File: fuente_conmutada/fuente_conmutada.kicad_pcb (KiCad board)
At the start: 2 copper layers, 206 x 163.7 mm, 64 parts, among them J1 shutdown, J2 Conn_01x03, J3 Conn_01x03, J4 Conn_01x02, J5 Conn_01x02, J6 in_red, J7 out_12v, J8 out_pwr, U1 UC3525

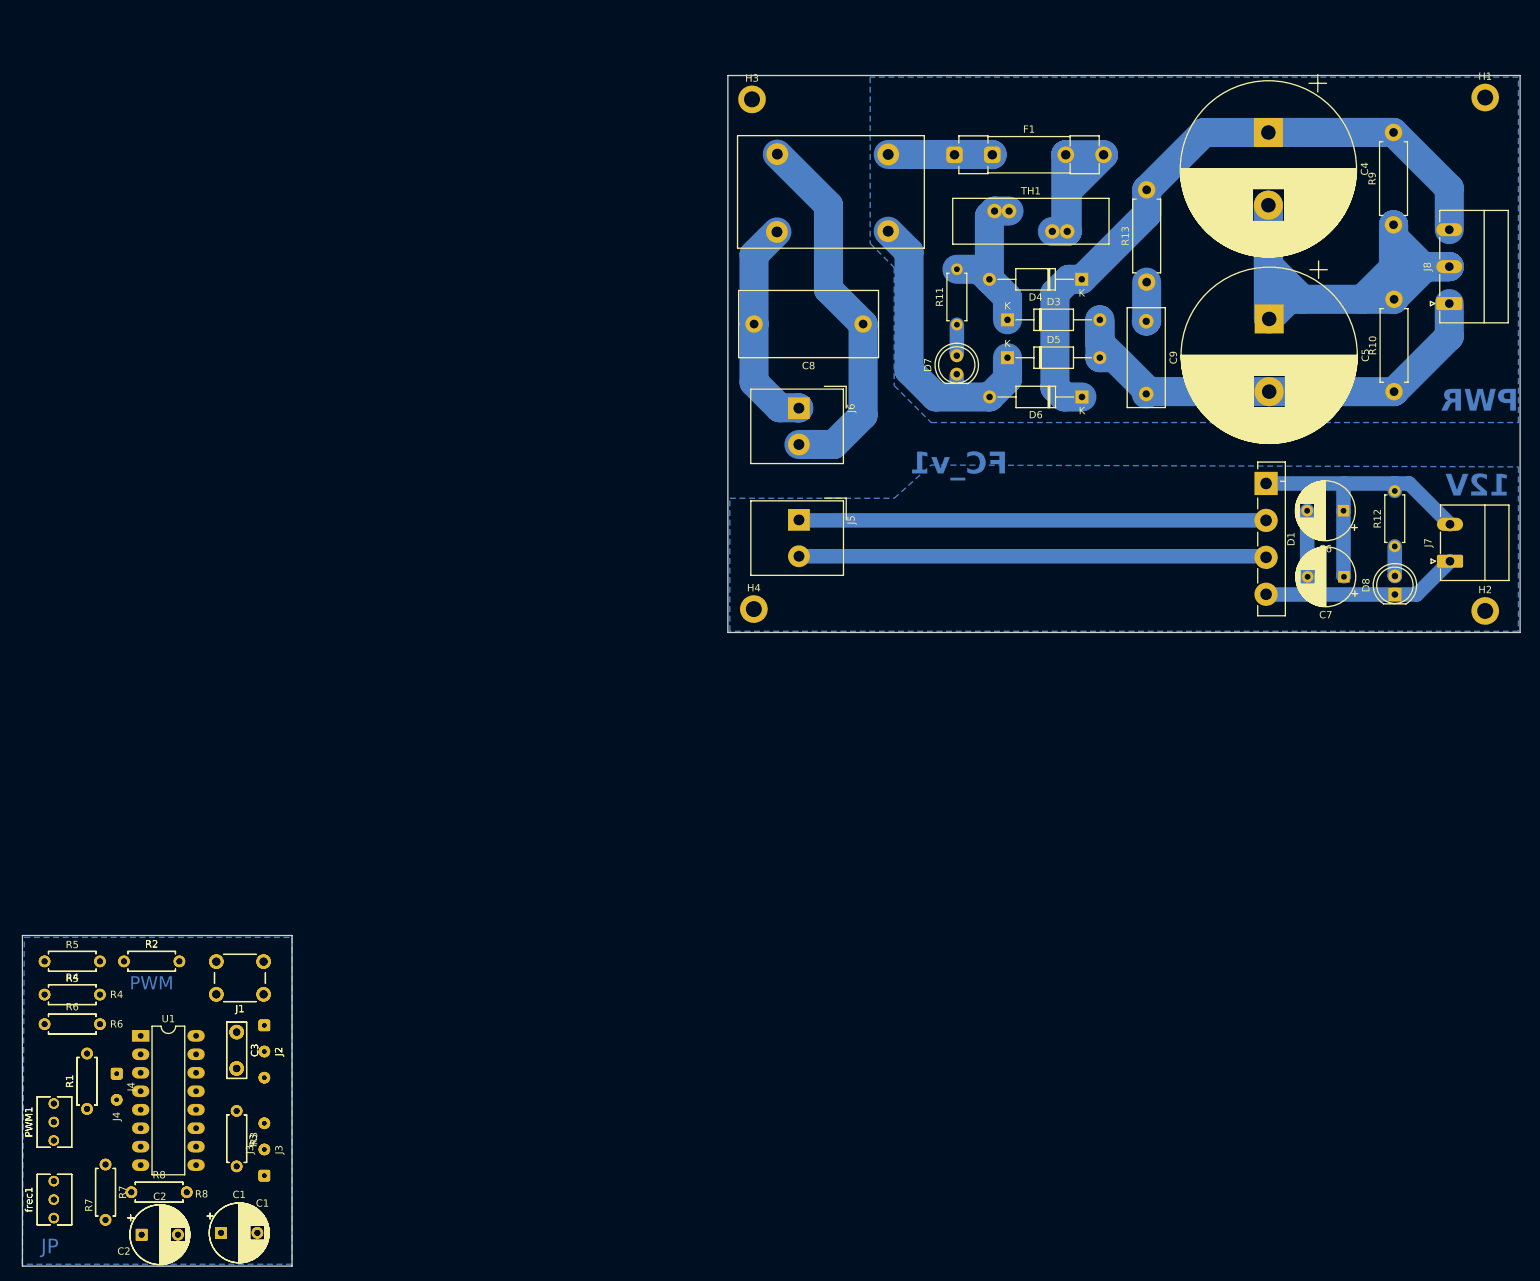
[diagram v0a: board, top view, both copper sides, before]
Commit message: fc_v1
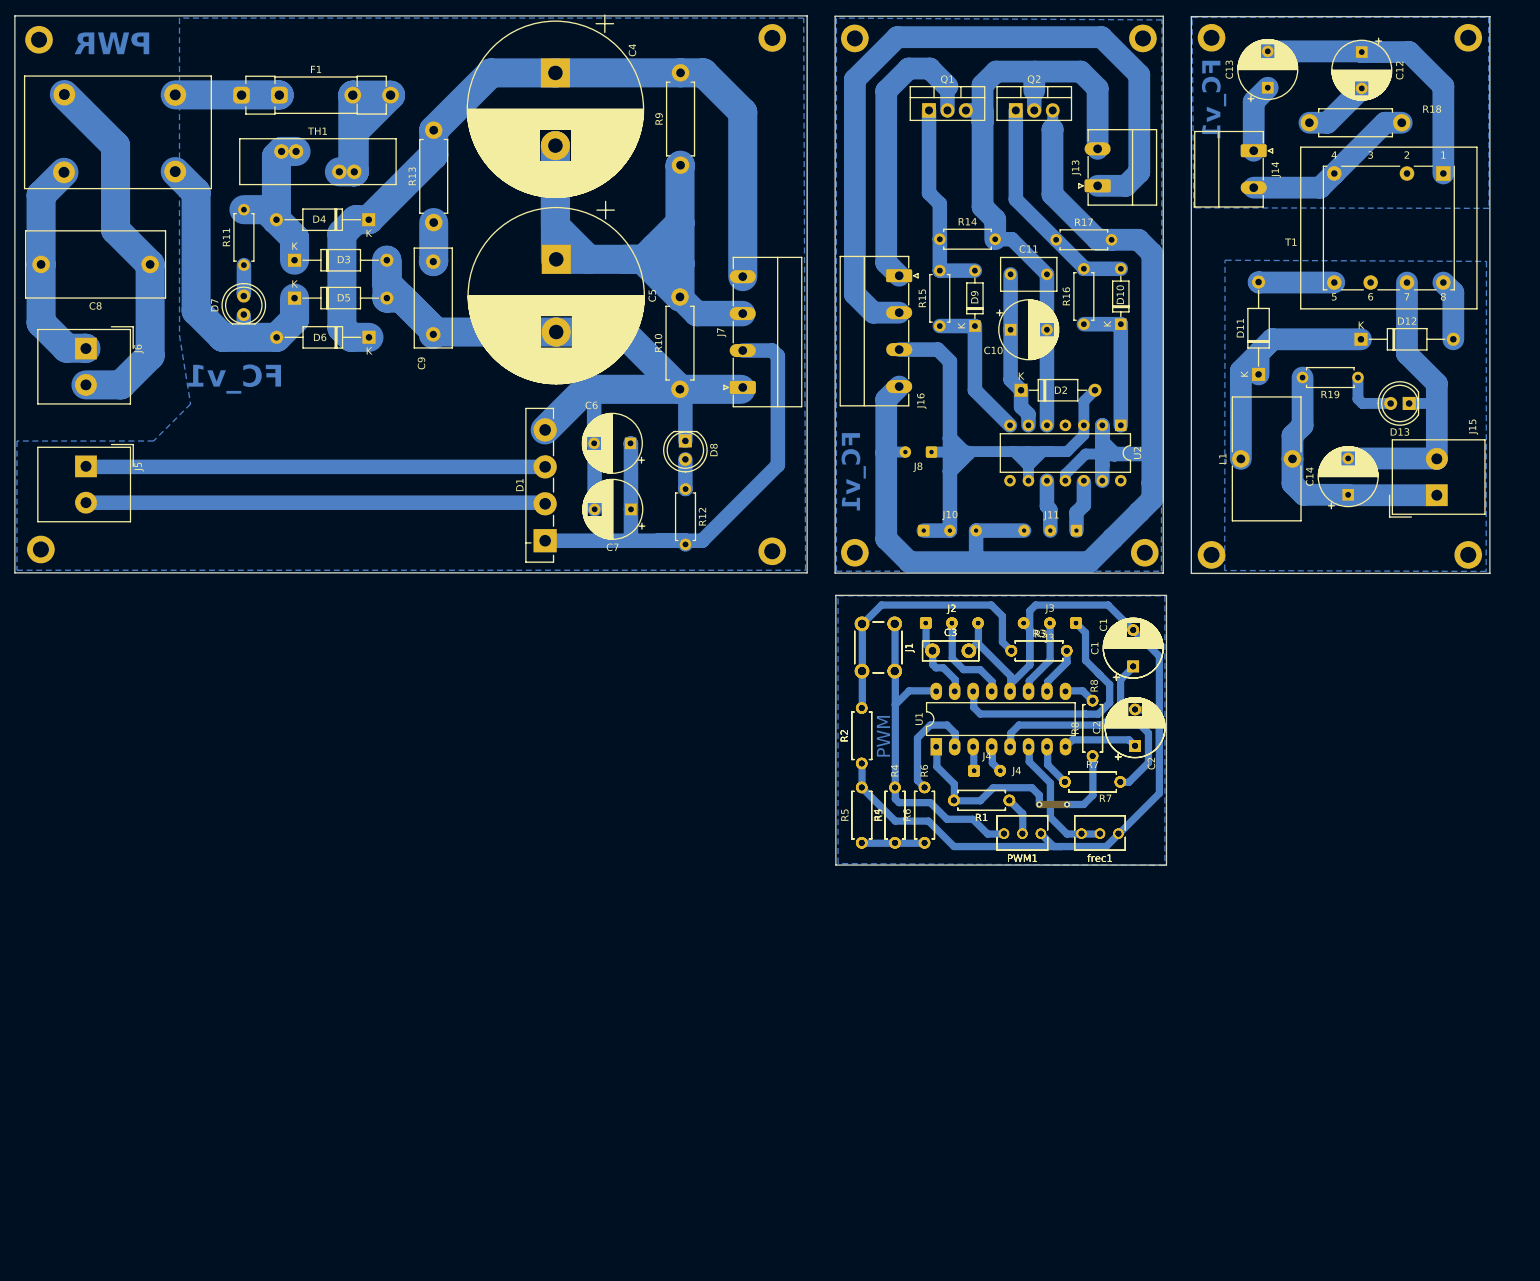
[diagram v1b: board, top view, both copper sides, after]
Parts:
- added C10: 100n, Capacitor_THT:CP_Radial_D8.0mm_P5.00mm, F.Cu at (156.2, 63.4)
- added C11: 22u, Capacitor_THT:C_Disc_D7.5mm_W4.4mm_P5.00mm, F.Cu at (156.2, 55.8)
- added C12: 100n, Capacitor_THT:CP_Radial_D8.0mm_P5.00mm, F.Cu at (204.5, 25.2)
- added C13: 100n, Capacitor_THT:CP_Radial_D8.0mm_P5.00mm, F.Cu at (191.6, 30.1)
- added C14: 100n, Capacitor_THT:CP_Radial_D8.0mm_P5.00mm, F.Cu at (202.6, 86.1)
- added D10: 1N4148, Diode_THT:D_DO-35_SOD27_P7.62mm_Horizontal, F.Cu at (171.4, 62.7)
- added D11: D, Diode_THT:D_A-405_P12.70mm_Horizontal, F.Cu at (190.3, 69.6)
- added D12: D, Diode_THT:D_A-405_P12.70mm_Horizontal, F.Cu at (204.4, 64.7)
- added D13: LED, LED_THT:LED_D5.0mm, F.Cu at (211.0, 73.6)
- added D2: D, Diode_THT:D_A-405_P10.16mm_Horizontal, F.Cu at (157.7, 71.8)
- added D9: 1N4148, Diode_THT:D_DO-35_SOD27_P7.62mm_Horizontal, F.Cu at (151.3, 62.9)
- added H10: MountingHole, MountingHole:MountingHole_2.2mm_M2_DIN965_Pad, F.Cu at (219.2, 23.3)
- added H11: MountingHole, MountingHole:MountingHole_2.2mm_M2_DIN965_Pad, F.Cu at (183.9, 94.4)
- added H12: MountingHole, MountingHole:MountingHole_2.2mm_M2_DIN965_Pad, F.Cu at (219.2, 94.4)
- added H5: MountingHole, MountingHole:MountingHole_2.2mm_M2_DIN965_Pad, F.Cu at (134.8, 94.1)
- added H6: MountingHole, MountingHole:MountingHole_2.2mm_M2_DIN965_Pad, F.Cu at (134.8, 23.4)
- added H7: MountingHole, MountingHole:MountingHole_2.2mm_M2_DIN965_Pad, F.Cu at (174.4, 23.4)
- added H8: MountingHole, MountingHole:MountingHole_2.2mm_M2_DIN965_Pad, F.Cu at (174.7, 94.1)
- added H9: MountingHole, MountingHole:MountingHole_2.2mm_M2_DIN965_Pad, F.Cu at (183.9, 23.3)
- added J10: pwm_power, Connector_Wire:SolderWire-0.1sqmm_1x03_P3.6mm_D0.4mm_OD1mm, F.Cu at (144.3, 91.1)
- added J11: pwm_señal, Connector_Wire:SolderWire-0.1sqmm_1x03_P3.6mm_D0.4mm_OD1mm, F.Cu at (165.3, 91.1)
- added J13: trafo, Connector_Phoenix_MC_HighVoltage:PhoenixContact_MC_1,5_2-G-5.08_1x02_P5.08mm_Horizontal, F.Cu at (168.2, 43.6)
- added J14: in_trafo, Connector_Phoenix_MC_HighVoltage:PhoenixContact_MC_1,5_2-G-5.08_1x02_P5.08mm_Horizontal, F.Cu at (189.7, 38.8)
- added J15: out_R, TerminalBlock_Altech:Altech_AK300_1x02_P5.00mm_45-Degree, F.Cu at (214.8, 86.2)
- added J16: in_pwr, Connector_Phoenix_MC_HighVoltage:PhoenixContact_MC_1,5_4-G-5.08_1x04_P5.08mm_Horizontal, F.Cu at (140.9, 56.0)
- added L1: L, Inductor_THT:L_Toroid_Vertical_L16.8mm_W9.2mm_P7.10mm_Vishay_TJ3, F.Cu at (187.9, 81.2)
- added Q1: IRF740, Package_TO_SOT_THT:TO-220-3_Vertical, F.Cu at (145.0, 33.3)
- added Q2: IRF740, Package_TO_SOT_THT:TO-220-3_Vertical, F.Cu at (156.9, 33.3)
- added R14: 1k, Resistor_THT:R_Axial_DIN0207_L6.3mm_D2.5mm_P7.62mm_Horizontal, F.Cu at (146.5, 51.0)
- added R15: 100, Resistor_THT:R_Axial_DIN0207_L6.3mm_D2.5mm_P7.62mm_Horizontal, F.Cu at (146.5, 62.9)
- added R16: 100, Resistor_THT:R_Axial_DIN0207_L6.3mm_D2.5mm_P7.62mm_Horizontal, F.Cu at (166.3, 62.7)
- added R17: 1k, Resistor_THT:R_Axial_DIN0207_L6.3mm_D2.5mm_P7.62mm_Horizontal, F.Cu at (162.5, 51.1)
- added R18: 150k, Resistor_THT:R_Axial_DIN0411_L9.9mm_D3.6mm_P12.70mm_Horizontal, F.Cu at (210.0, 35.0)
- added R19: 22k, Resistor_THT:R_Axial_DIN0207_L6.3mm_D2.5mm_P7.62mm_Horizontal, F.Cu at (204.0, 70.0)
- added T1: Transformer_1P_SS, Transformer_THT:Transformer_Breve_TEZ-22x24, F.Cu at (215.7, 41.9)
- added U2: IR2110, Package_DIP:DIP-14_W7.62mm, F.Cu at (171.4, 76.6)
- J7: value out_12v -> in_pwr; footprint Connector_Phoenix_MC_HighVoltage:PhoenixContact_MC_1,5_2-G-5.08_1x02_P5.08mm_Horizontal -> Connector_Phoenix_MC_HighVoltage:PhoenixContact_MC_1,5_4-G-5.08_1x04_P5.08mm_Horizontal
- J8: value out_pwr -> fan; footprint Connector_Phoenix_MC_HighVoltage:PhoenixContact_MC_1,5_3-G-5.08_1x03_P5.08mm_Horizontal -> Connector_Wire:SolderWire-0.1sqmm_1x02_P3.6mm_D0.4mm_OD1mm
- moved C2 152.3 mm to (173.3, 120.7), turned to 90 degrees (x2)
- moved frec1 149.2 mm to (166.0, 132.7), turned to 180 degrees (x2)
- moved C1 147.7 mm to (173.1, 109.7), turned to 90 degrees (x2)
- moved R8 145.2 mm to (167.5, 122.1), turned to 90 degrees (x2)
- moved R7 142.1 mm to (163.7, 125.6), turned to 0 degrees (x2)
- moved PWM1 135.8 mm to (155.3, 132.7), turned to 180 degrees (x2)
- moved J3 135.1 mm to (165.2, 103.8), turned to 180 degrees
- moved J3 135.0 mm to (165.2, 103.8), turned to 180 degrees
- moved R1 133.8 mm to (156.1, 128.2), turned to 180 degrees
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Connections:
- C3 pad 1: +12V -> Vc
- C5 pad 2: GNDPWR -> GND
- C6 pad 1: +12V -> Vc
- C7 pad 1: +12V -> Vc
- C9 pad 2: GNDPWR -> GND
- D1 pad 1: +12V -> Vc
- D1 pad 2: Net-(J5-Pin_1) -> Net-(J5-Pin_2)
- D1 pad 3: Net-(J5-Pin_2) -> Net-(J5-Pin_1)
- D3 pad 2: GNDPWR -> GND
- D5 pad 2: GNDPWR -> GND
- J2 pad 1: +12V -> Vc
- J7 pad 2: +12V -> Vc
- J8 pad 1: GNDPWR -> Vc
- J8 pad 2: 155V -> GND
- R10 pad 1: GNDPWR -> GND
- R12 pad 2: +12V -> Vc
- U1 pad 15: +12V -> Vc
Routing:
- net GND: track 38.7 -> 420.4 mm
- net Vc: track 0.00 -> 166.1 mm
- net 155V: track 108.8 -> 218.4 mm
- net VS: track 0.00 -> 96.4 mm
- net GNDPWR: track 76.0 -> 0.00 mm
- net 310V: track 91.5 -> 148.5 mm
- net Vref: track 0.00 -> 47.5 mm
- net OutB: track 0.00 -> 42.5 mm
- net GNDREF: track 0.00 -> 42.3 mm
- net Net-(U1-CT): track 0.00 -> 41.0 mm
- net Net-(T1-AA): track 0.00 -> 38.1 mm
- net Net-(J1-Pin_2): track 0.00 -> 37.9 mm
- net Net-(D11-K): track 0.00 -> 36.0 mm
- net Net-(U1-INV): track 0.00 -> 35.9 mm, vias 0 -> 2
- net Net-(J15-Pin_1): track 0.00 -> 35.7 mm
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- added copper zone on B.Cu, net (none)
- added copper zone on B.Cu, net GNDREF
- removed copper zone on B.Cu, net GNDPWR
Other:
- board size 206 x 163.7 mm -> 202.9 x 116.8 mm
- board text removed: "12V"
- board text removed: "JP"
